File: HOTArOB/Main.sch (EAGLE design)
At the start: 15 parts

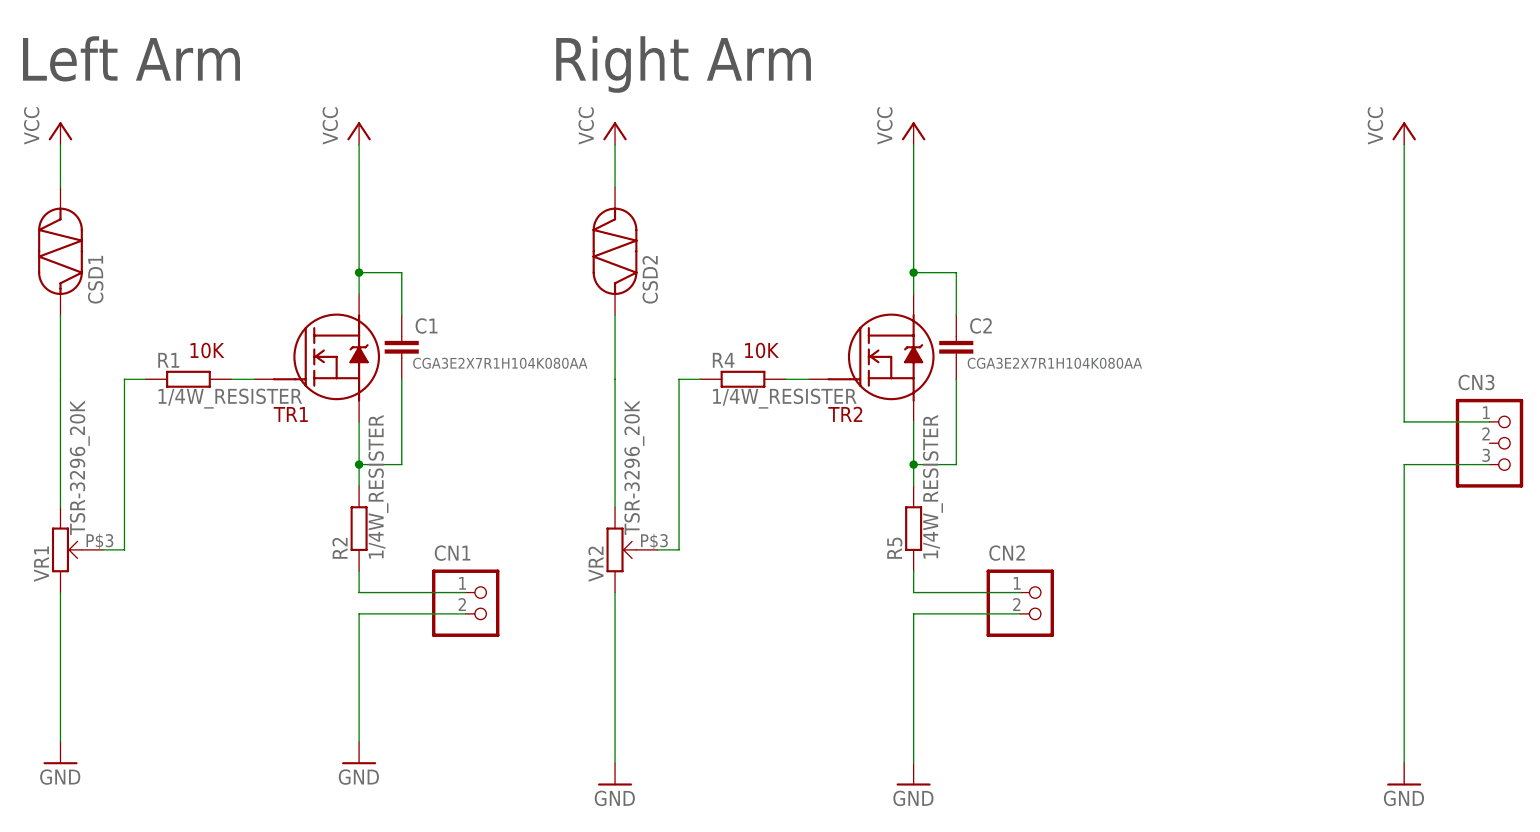
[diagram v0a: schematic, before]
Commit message: working commit
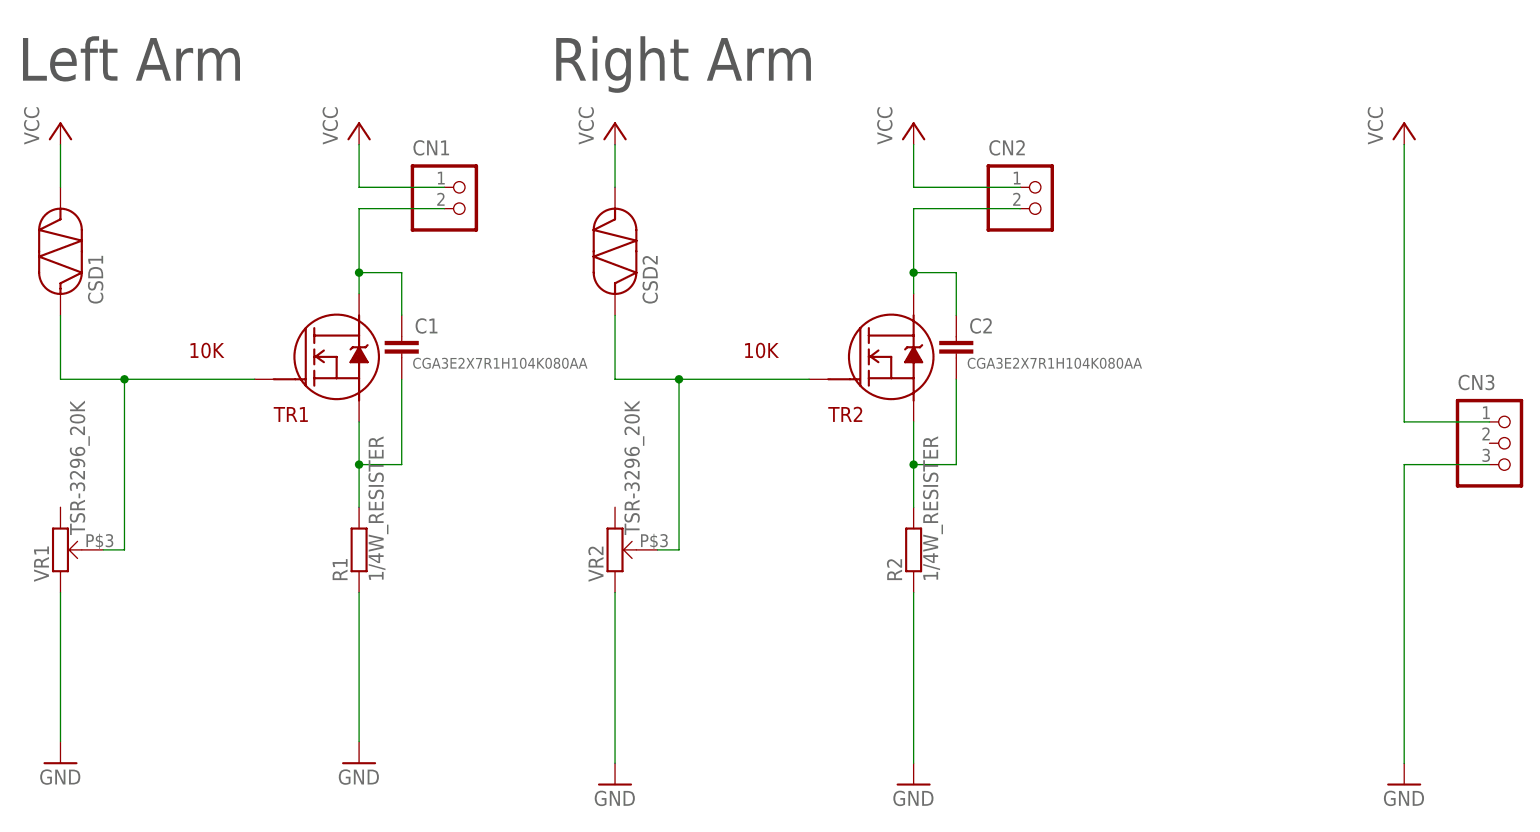
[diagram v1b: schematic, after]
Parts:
- removed R4, R5: 1/4W_RESISTER, Tr_EXT:1/4W_RESISTER
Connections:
- removed net N$10: R4.2, VR2.P$1
- removed net N$5: CN1.1, R2.2
- removed net N$6: CN2.1, R5.2
- removed net N$7: CSD2.P$1, VR2.1
- net GND: now also R1.2, R2.2; no longer CN1.2, CN2.2
- net N$1: now also C1.1, CN1.2, TR1.D; no longer R1.1, TR1.G
- net N$2: now also R1.1; no longer R2.1
- net N$3: now also C2.1, CN2.2, TR2.D; no longer CSD1.P$1, VR1.1
- net N$4: now also R2.1; no longer R5.1
- net N$8: now also CSD2.P$1, VR2.P$1; no longer R4.1
- net N$9: now also CSD1.P$1, TR1.G; no longer R1.2
- net VCC: now also CN1.1, CN2.1; no longer C1.1, C2.1, TR1.D, TR2.D
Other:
- moved on the sheet: CN1, CN2, R1, R2
